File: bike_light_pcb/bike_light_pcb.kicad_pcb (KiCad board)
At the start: 2 copper layers, 55.9 x 25.4 mm, 7 parts, among them J1 Conn_01x03_Male, J2 Conn_01x04_Female, J3 Conn_01x02_Female, U1 Teensy4.0, U2 HM18_BLE, U3 MPU605, U4 charge_module

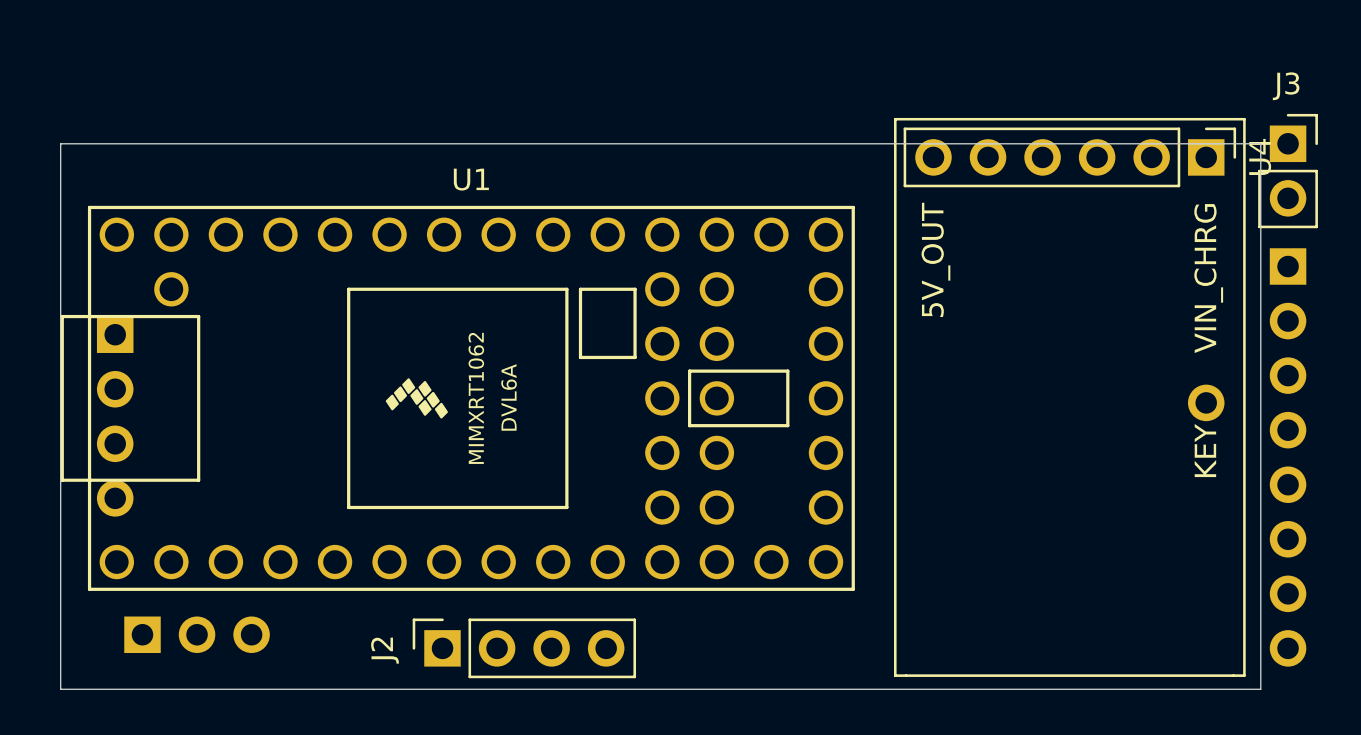
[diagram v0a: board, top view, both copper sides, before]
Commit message: draft of general layout
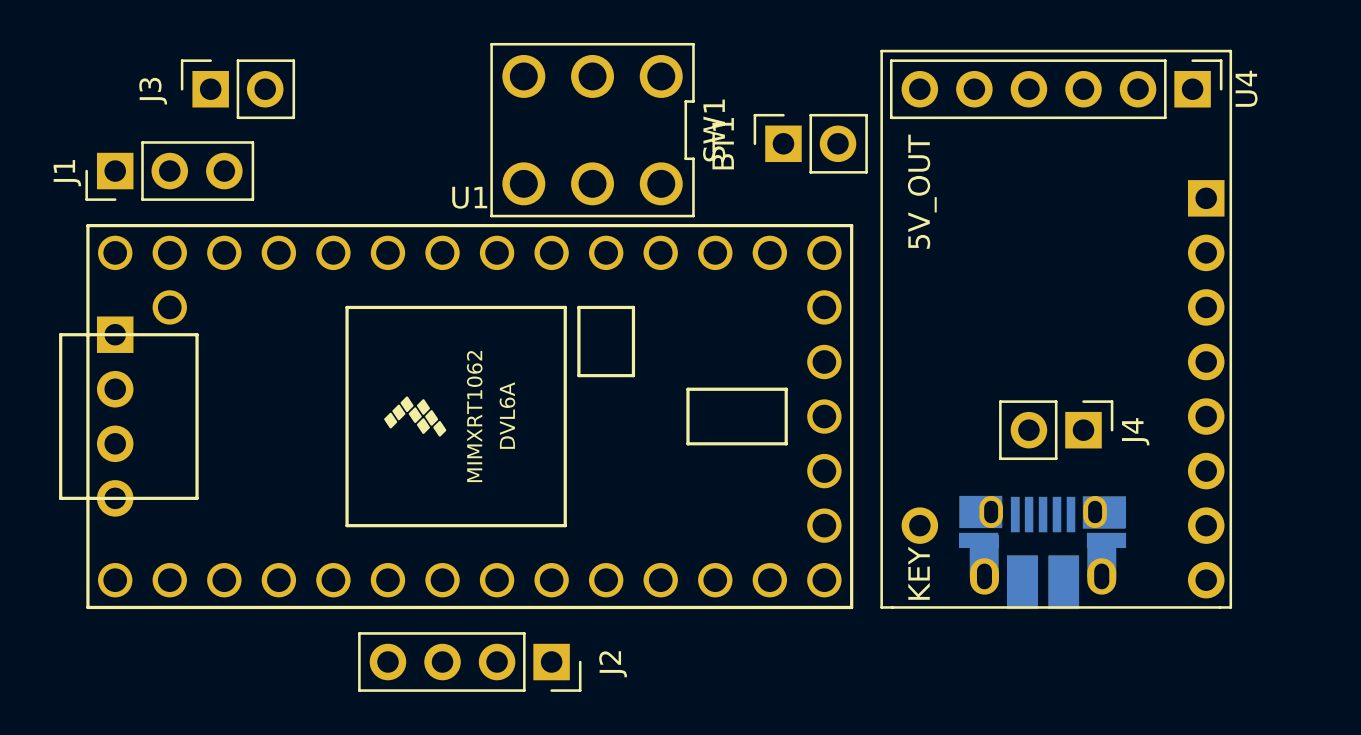
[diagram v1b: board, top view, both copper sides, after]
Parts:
- added BT1: Battery_Cell, Connector_PinSocket_2.54mm:PinSocket_1x02_P2.54mm_Vertical, F.Cu at (140.3, 50.8)
- added J4: Conn_01x02_Female, Connector_PinHeader_2.54mm:PinHeader_1x02_P2.54mm_Vertical, F.Cu at (154.3, 64.1)
- added J5: USB_B_Micro_Charge, Connector_USB:USB_Micro-B_Amphenol_10103594-0001LF_Horizontal, B.Cu at (152.4, 69.8)
- added SW1: SW_Push_DPDT, custom_footprints:SLIDE_SW_OS202013MT8QN1, F.Cu at (131.4, 50.2)
- J1: moved to F.Cu
- moved J3 50.2 mm to (113.7, 48.3), turned to 90 degrees
- moved J1 21.6 mm to (109.2, 52.1), turned to 90 degrees
- moved U3 13.9 mm to (160.0, 53.3)
- moved J2 5.12 mm to (129.5, 74.9), turned to 270 degrees
- moved U4 3.24 mm to (159.4, 48.3)
- moved U1 0.85 mm to (125.7, 63.5)
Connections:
- J1 pad 1: Net-(J1-Pad1) -> 5V_MAIN
- J1 pad 2: Net-(J1-Pad2) -> RGB_D
- J1 pad 3: Net-(J1-Pad3) -> GND_MAIN
- J3 pad 1: Net-(J3-Pad1) -> 5V_MAIN
- J3 pad 2: Net-(J3-Pad2) -> GND_MAIN
- U1 pad 10: Net-(U1-Pad10) -> Net-(J2-Pad1)
- U1 pad 11: Net-(U1-Pad11) -> CHRG_KEY
- U1 pad 17: Net-(U1-Pad17) -> GND_MAIN
- U1 pad 27: Net-(U1-Pad27) -> RGB_D
- U1 pad 32: Net-(U1-Pad32) -> GND_MAIN
- U1 pad 34: Net-(U1-Pad34) -> TEENSY_VUSB
- U1 pad 6: Net-(U1-Pad6) -> Net-(J2-Pad4)
- U1 pad 7: Net-(U1-Pad7) -> Net-(J2-Pad3)
- U1 pad 9: Net-(U1-Pad9) -> Net-(J2-Pad2)
- U2 pad 1: Net-(U2-Pad1) -> 5V_MAIN
- U2 pad 2: Net-(U2-Pad2) -> GND_MAIN
- U2 pad 3: Net-(U2-Pad3) -> Net-(U1-Pad3)
- U2 pad 4: Net-(U2-Pad4) -> Net-(U1-Pad2)
- U3 pad 1: Net-(U3-Pad1) -> 5V_MAIN
- U3 pad 2: Net-(U3-Pad2) -> GND_MAIN
- U3 pad 3: Net-(U3-Pad3) -> Net-(U1-Pad26)
- U3 pad 4: Net-(U3-Pad4) -> Net-(U1-Pad25)
- U3 pad 8: Net-(U3-Pad8) -> Net-(U1-Pad22)
- U4 pad 1: Net-(U4-Pad1) -> 5V_CHRG
- U4 pad 2: Net-(U4-Pad2) -> GND_CHRG
- U4 pad 5: Net-(U4-Pad5) -> GND_MODULE
- U4 pad 6: Net-(U4-Pad6) -> 5V_MODULE
- U4 pad 7: Net-(U4-Pad7) -> CHRG_KEY
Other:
- board outline removed
